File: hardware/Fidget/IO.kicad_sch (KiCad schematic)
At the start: 24 parts, among them J4 EXT I/O, J5 SPI2, J6 USART1, J7 I^{2}C1, J8 USART2, SW2 UB1, SW3 UB1, U2 ICE40HX4K-TQ144

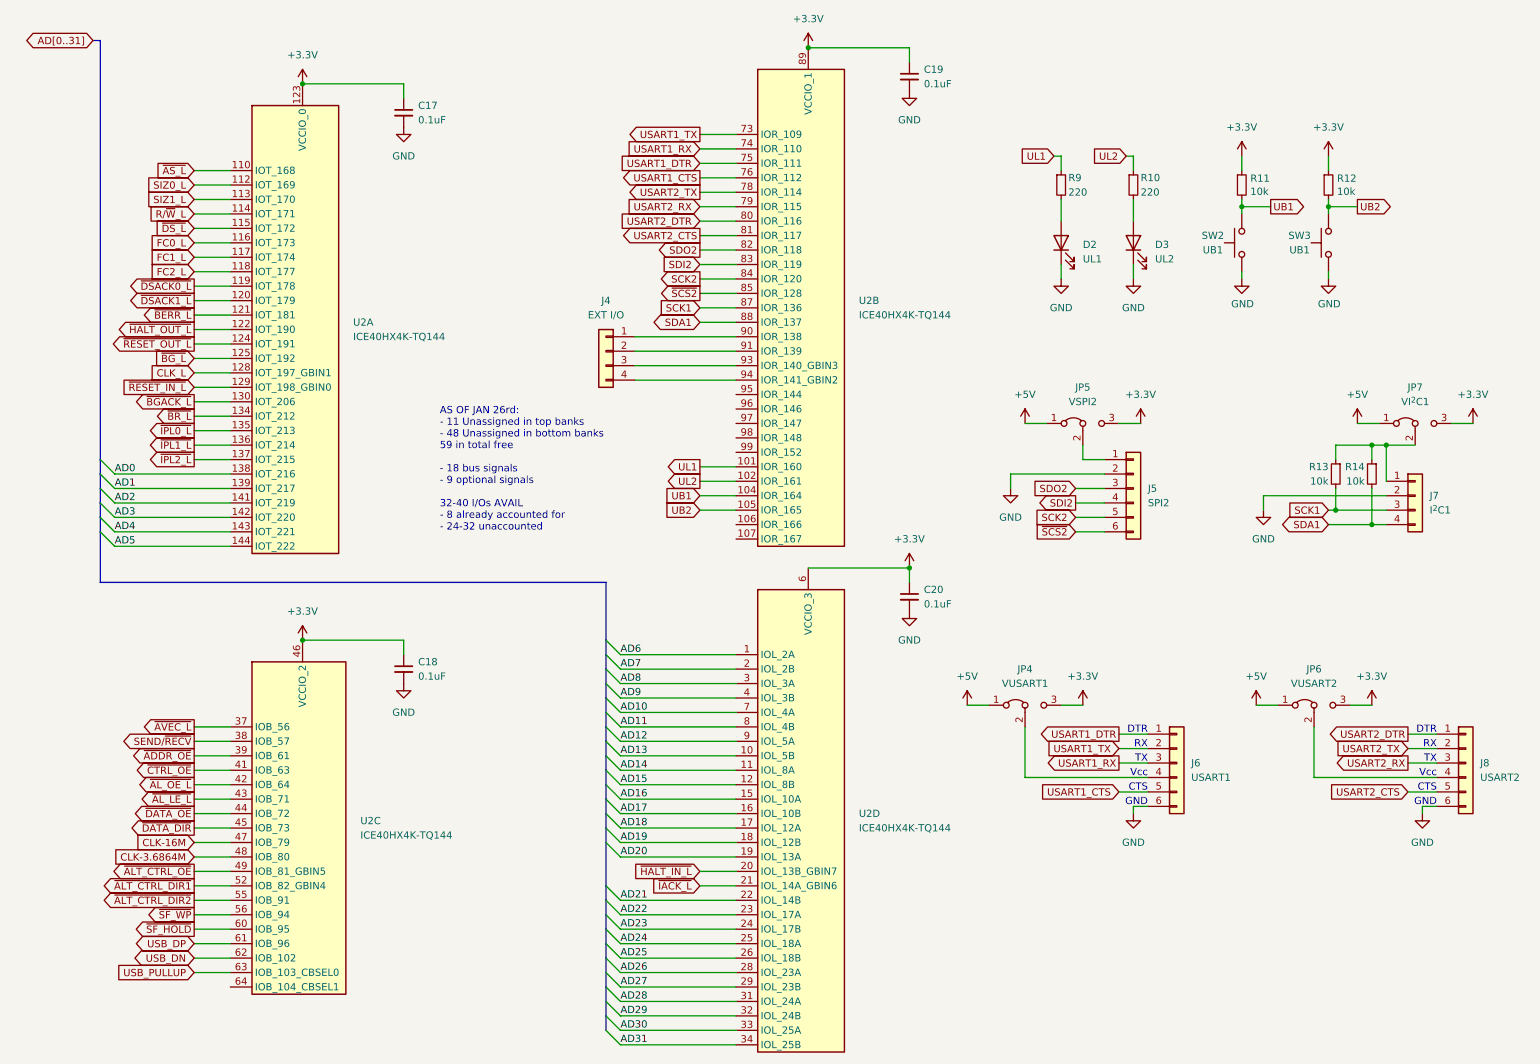
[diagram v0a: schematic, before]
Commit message: Almost done Rev1 board design
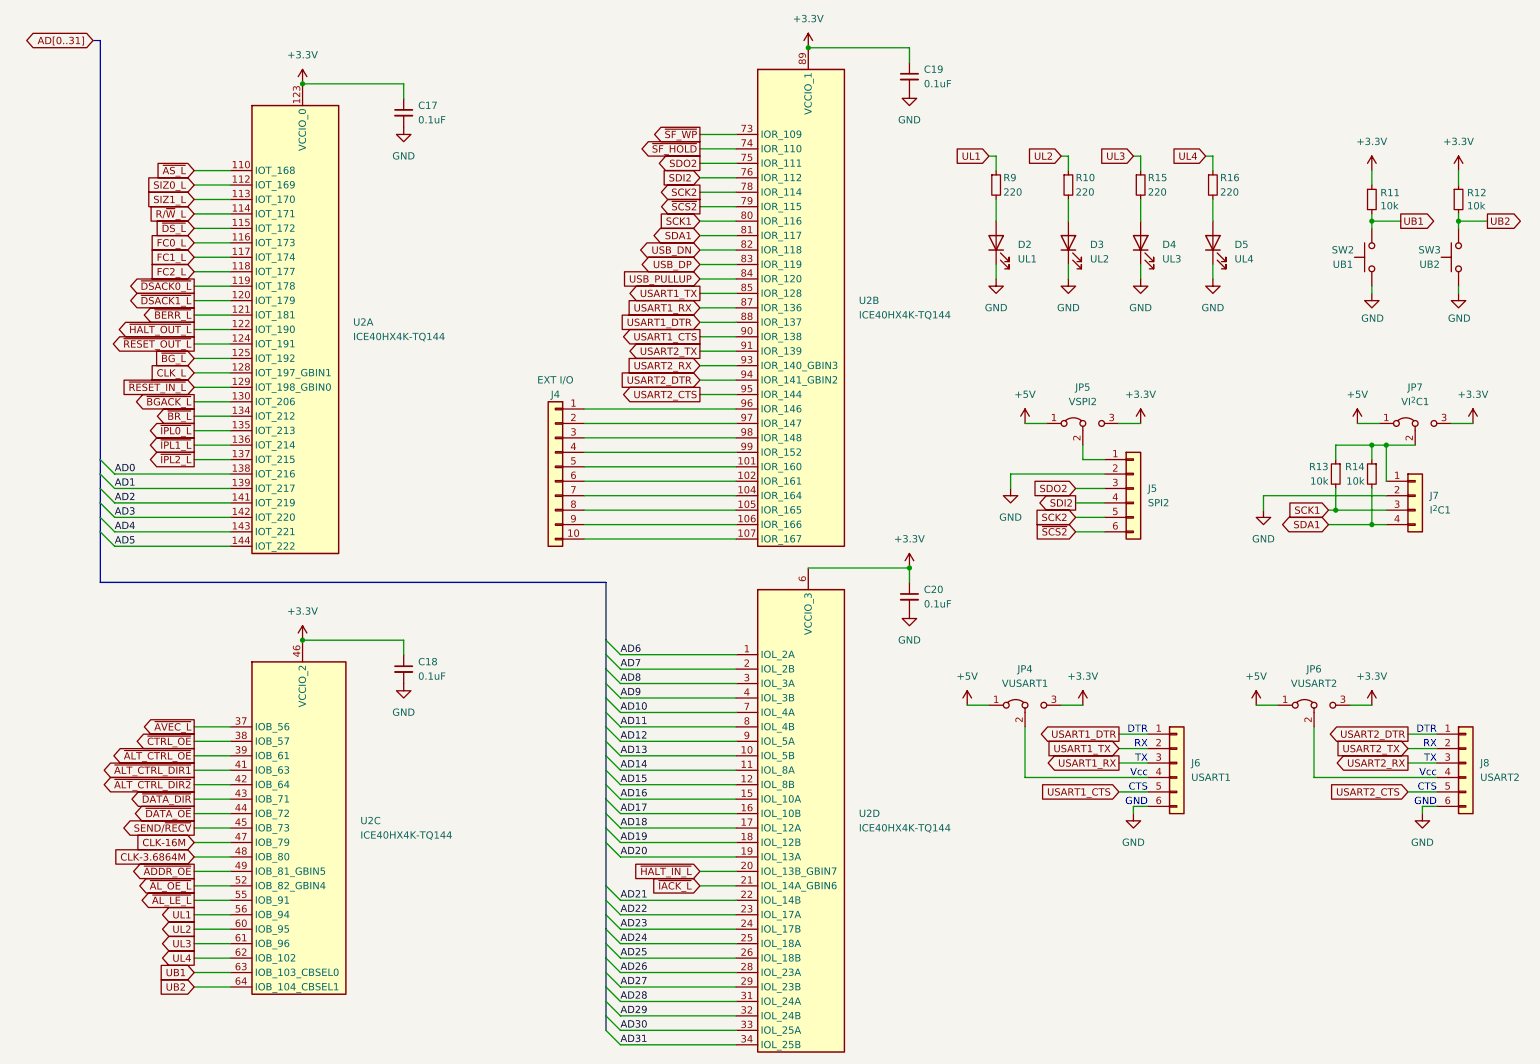
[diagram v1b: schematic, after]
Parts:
- added D4: UL3, LED_SMD:LED_PLCC-2_3.4x3.0mm_KA, symbol Device:LED
- added D5: UL4, LED_SMD:LED_PLCC-2_3.4x3.0mm_KA, symbol Device:LED
- added R15, R16: 220, Resistor_SMD:R_0805_2012Metric_Pad1.20x1.40mm_HandSolder, symbol Device:R_Small
- D2, D3: footprint (none) -> LED_SMD:LED_PLCC-2_3.4x3.0mm_KA
- J4: footprint Connector_PinHeader_2.54mm:PinHeader_1x04_P2.54mm_Vertical -> Connector_PinHeader_2.54mm:PinHeader_2x05_P2.54mm_Vertical; symbol Connector_Generic:Conn_01x04 -> Connector_Generic:Conn_01x10
- R10, R11, R12, R13, R14, R9: footprint Resistor_THT:R_Axial_DIN0204_L3.6mm_D1.6mm_P5.08mm_Horizontal -> Resistor_SMD:R_0805_2012Metric_Pad1.20x1.40mm_HandSolder
- SW3: value UB1 -> UB2
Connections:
- net GND: now also D4.1 (K), D5.1 (K)
- net SCK1: now also U2.80 (IOR_116); no longer U2.87 (IOR_136)
- net SCK2: now also U2.78 (IOR_114); no longer U2.84 (IOR_120)
- net SDA1: now also U2.81 (IOR_117); no longer U2.88 (IOR_137)
- net SDI2: now also U2.76 (IOR_112); no longer U2.83 (IOR_119)
- net SDO2: now also U2.75 (IOR_111); no longer U2.82 (IOR_118)
- net SEND/~{RECV}: now also U2.45 (IOB_73); no longer U2.38 (IOB_57)
- net UB1: now also U2.63 (IOB_103_CBSEL0); no longer U2.104 (IOR_164)
- net UB2: now also U2.64 (IOB_104_CBSEL1); no longer U2.105 (IOR_165)
- net UL1: now also U2.56 (IOB_94); no longer U2.101 (IOR_160)
- net UL2: now also U2.60 (IOB_95); no longer U2.102 (IOR_161)
- net USART1_CTS: now also U2.90 (IOR_138); no longer U2.76 (IOR_112)
- net USART1_DTR: now also U2.88 (IOR_137); no longer U2.75 (IOR_111)
- net USART1_RX: now also U2.87 (IOR_136); no longer U2.74 (IOR_110)
- net USART1_TX: now also U2.85 (IOR_128); no longer U2.73 (IOR_109)
- net USART2_CTS: now also U2.95 (IOR_144); no longer U2.81 (IOR_117)
- net USART2_DTR: now also U2.94 (IOR_141_GBIN2); no longer U2.80 (IOR_116)
- net USART2_RX: now also U2.93 (IOR_140_GBIN3); no longer U2.79 (IOR_115)
- net USART2_TX: now also U2.91 (IOR_139); no longer U2.78 (IOR_114)
- net USB_DN: now also U2.82 (IOR_118); no longer U2.62 (IOB_102)
- net USB_DP: now also U2.83 (IOR_119); no longer U2.61 (IOB_96)
- net USB_PULLUP: now also U2.84 (IOR_120); no longer U2.63 (IOB_103_CBSEL0)
- net ~{ADDR_OE}: now also U2.49 (IOB_81_GBIN5); no longer U2.39 (IOB_61)
- net ~{ALT_CTRL_DIR1}: now also U2.41 (IOB_63); no longer U2.52 (IOB_82_GBIN4)
- net ~{ALT_CTRL_DIR2}: now also U2.42 (IOB_64); no longer U2.55 (IOB_91)
- net ~{ALT_CTRL_OE}: now also U2.39 (IOB_61); no longer U2.49 (IOB_81_GBIN5)
- net ~{AL_LE_L}: now also U2.55 (IOB_91); no longer U2.43 (IOB_71)
- net ~{AL_OE_L}: now also U2.52 (IOB_82_GBIN4); no longer U2.42 (IOB_64)
- net ~{CTRL_OE}: now also U2.38 (IOB_57); no longer U2.41 (IOB_63)
- net ~{DATA_DIR}: now also U2.43 (IOB_71); no longer U2.45 (IOB_73)
- net ~{SCS2}: now also U2.79 (IOR_115); no longer U2.85 (IOR_128)
- net ~{SF_HOLD}: now also U2.74 (IOR_110); no longer U2.60 (IOB_95)
- net ~{SF_WP}: now also U2.73 (IOR_109); no longer U2.56 (IOB_94)
- net at U2.106 (IOR_166): now also J4.9 (Pin_9)
- net at U2.107 (IOR_167): now also J4.10 (Pin_10)
- net at J4.1 (Pin_1): now also U2.96 (IOR_146); no longer U2.90 (IOR_138)
- net at J4.2 (Pin_2): now also U2.97 (IOR_147); no longer U2.91 (IOR_139)
- net at J4.3 (Pin_3): now also U2.98 (IOR_148); no longer U2.93 (IOR_140_GBIN3)
- net at J4.4 (Pin_4): now also U2.99 (IOR_152); no longer U2.94 (IOR_141_GBIN2)
- new net: D4.2 (A), R15.2
- new net: D5.2 (A), R16.2
- new net: J4.5 (Pin_5), U2.101 (IOR_160)
- new net: J4.6 (Pin_6), U2.102 (IOR_161)
- new net: J4.7 (Pin_7), U2.104 (IOR_164)
- new net: J4.8 (Pin_8), U2.105 (IOR_165)
- new net UL3: R15.1, U2.61 (IOB_96)
- new net UL4: R16.1, U2.62 (IOB_102)
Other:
- note removed: "AS OF JAN 26rd: - 11 Unassigned in top banks - 48 Unassigned in bottom banks 59 in total free - 18 bus signals - 9 optional signals 32-40 I/Os AVAIL - 8 already accounted for - 24-32 unaccounted"
- moved on the sheet: D2, D3, R10, R11, R12, R9, SW2, SW3
